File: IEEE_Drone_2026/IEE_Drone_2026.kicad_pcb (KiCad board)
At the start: 4 copper layers, 44.9 x 45.5 mm, 44 parts, among them IC1 TPSM84209RKHT, J1 ESC, J13 USB_C_Receptacle_USB2.0_16P, J2 M4 Mounting, J3 M4 Mounting, J4 M4 Mounting, J5 M4 Mounting, U2 STM32F405RGTx, U3 BMP390, U5 LIS2MDL, Y2 ABMM2-32.768MHZ-E2F-T

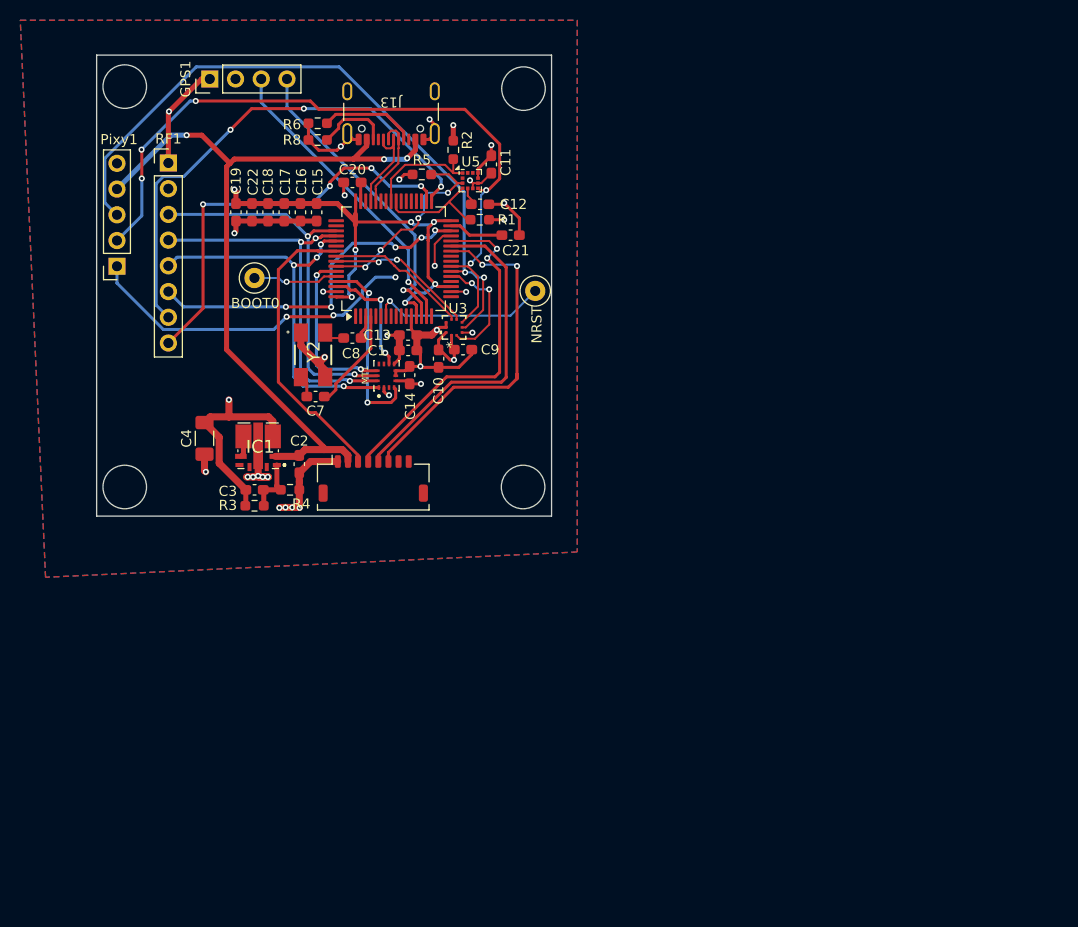
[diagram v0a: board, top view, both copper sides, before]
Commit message: complete redesign
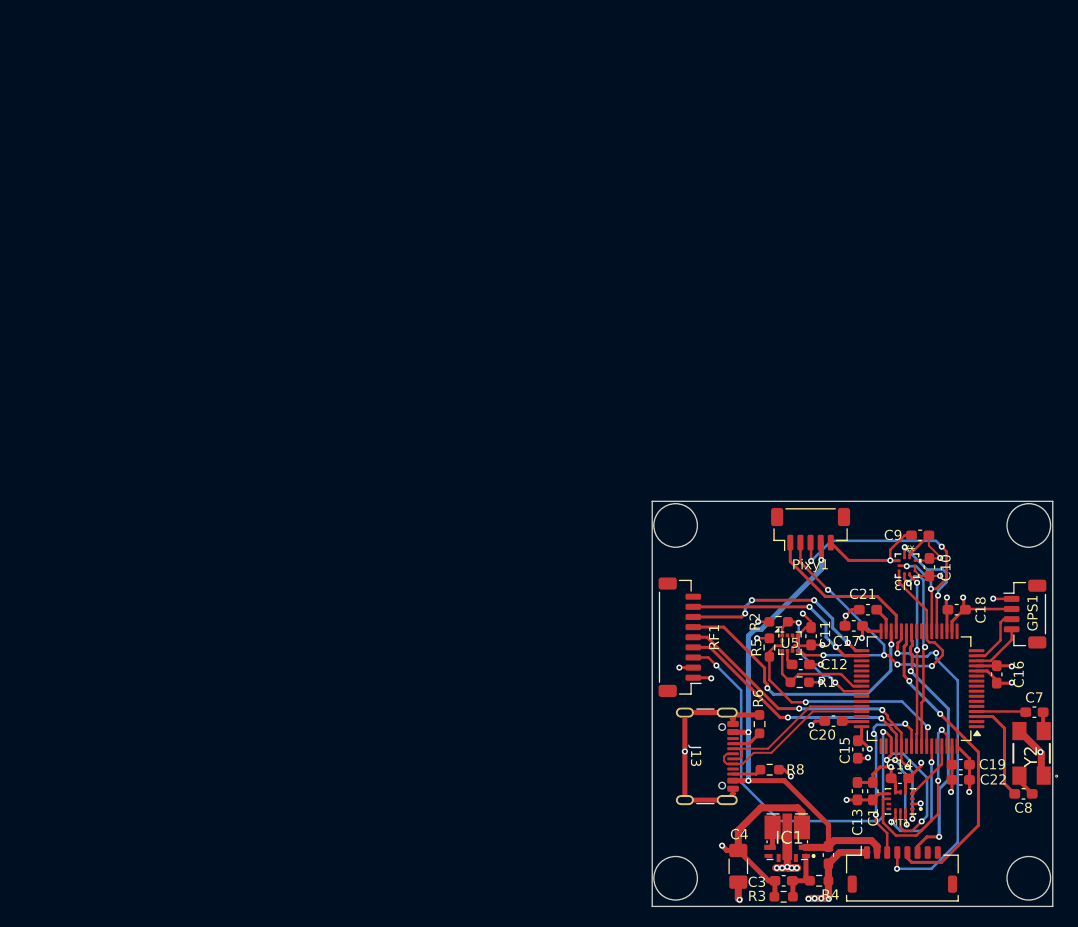
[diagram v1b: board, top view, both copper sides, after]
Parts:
- removed BOOT0, NRST: TestPoint, TestPoint:TestPoint_Loop_D2.50mm_Drill1.0mm
- GPS1: footprint Connector_PinHeader_2.54mm:PinHeader_1x04_P2.54mm_Vertical -> Connector_JST:JST_SH_BM04B-SRSS-TB_1x04-1MP_P1.00mm_Vertical
- Pixy1: footprint Connector_PinSocket_2.54mm:PinSocket_1x05_P2.54mm_Vertical -> Connector_JST:JST_SH_BM05B-SRSS-TB_1x05-1MP_P1.00mm_Vertical
- RF1: footprint Connector_PinHeader_2.54mm:PinHeader_1x08_P2.54mm_Vertical -> Connector_JST:JST_SH_BM09B-SRSS-TB_1x09-1MP_P1.00mm_Vertical
- moved GPS1 96.3 mm to (156.7, 138.6), turned to -90 degrees
- moved C19 90.0 mm to (150.4, 153.5), turned to 180 degrees
- moved C22 89.7 mm to (150.4, 155.0), turned to 180 degrees
- moved C16 82.5 mm to (153.9, 144.6)
- moved Y2 81.1 mm to (157.4, 152.4), turned to 90 degrees
- moved C8 80.1 mm to (156.6, 156.4), turned to 180 degrees
- moved C18 78.5 mm to (150.0, 138.2), turned to 0 degrees
- moved C7 77.5 mm to (157.6, 148.3), turned to 180 degrees
- moved R8 76.5 mm to (131.5, 154.0), turned to 180 degrees
- moved C15 75.3 mm to (140.2, 152.0)
- moved R6 73.6 mm to (130.5, 149.5), turned to -90 degrees
- moved Pixy1 73.2 mm to (135.5, 130.3), turned to 0 degrees
- moved C20 71.3 mm to (137.8, 149.2)
- moved J13 71.3 mm to (124.2, 152.7), turned to -90 degrees
- moved J3 69.5 mm to (122.2, 129.9)
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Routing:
- net +3.3V: track 103.1 -> 64.6 mm, vias 16 -> 15
- net /MISO: track 67.9 -> 29.9 mm, vias 2 -> 4
- net /MOSI: track 71.7 -> 40.5 mm
- net /PB12: track 50.3 -> 20.3 mm, vias 3 -> 4
- net +VDC: track 77.7 -> 50.2 mm
- net /SCK: track 41.9 -> 16.1 mm, vias 4 -> 0
- net /TX: track 30.5 -> 5.37 mm, vias 1 -> 0
- net /RX: track 30.2 -> 6.00 mm, vias 1 -> 0
- net GND: track 76.6 -> 98.1 mm, vias 23 -> 26
- net /PB13: track 40.8 -> 19.4 mm, vias 4 -> 2
- net /PB3: track 40.1 -> 18.7 mm, vias 0 -> 3
- net /SCK (SPI3): track 37.8 -> 56.8 mm, vias 2 -> 4
- net Net-(U2-NRST): track 17.6 -> 0.00 mm, vias 1 -> 0
- net /PB8: track 18.7 -> 5.91 mm, vias 2 -> 0
- net /PB0: track 35.3 -> 25.6 mm
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- added copper zone on In1.Cu, net +3.3V
- removed copper zone on B.Cu, net GND
- removed copper zone on F.Cu, net GND
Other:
- board size 44.9 x 45.5 mm -> 39.5 x 40 mm
